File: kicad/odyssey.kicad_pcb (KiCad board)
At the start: 2 copper layers, 33.6 x 18 mm, 7 parts, among them U1 ALS31313KLEATR, U2 MPU-6050, U3 MS560702BA03-50, U4 RP2040, U5 TF-01A

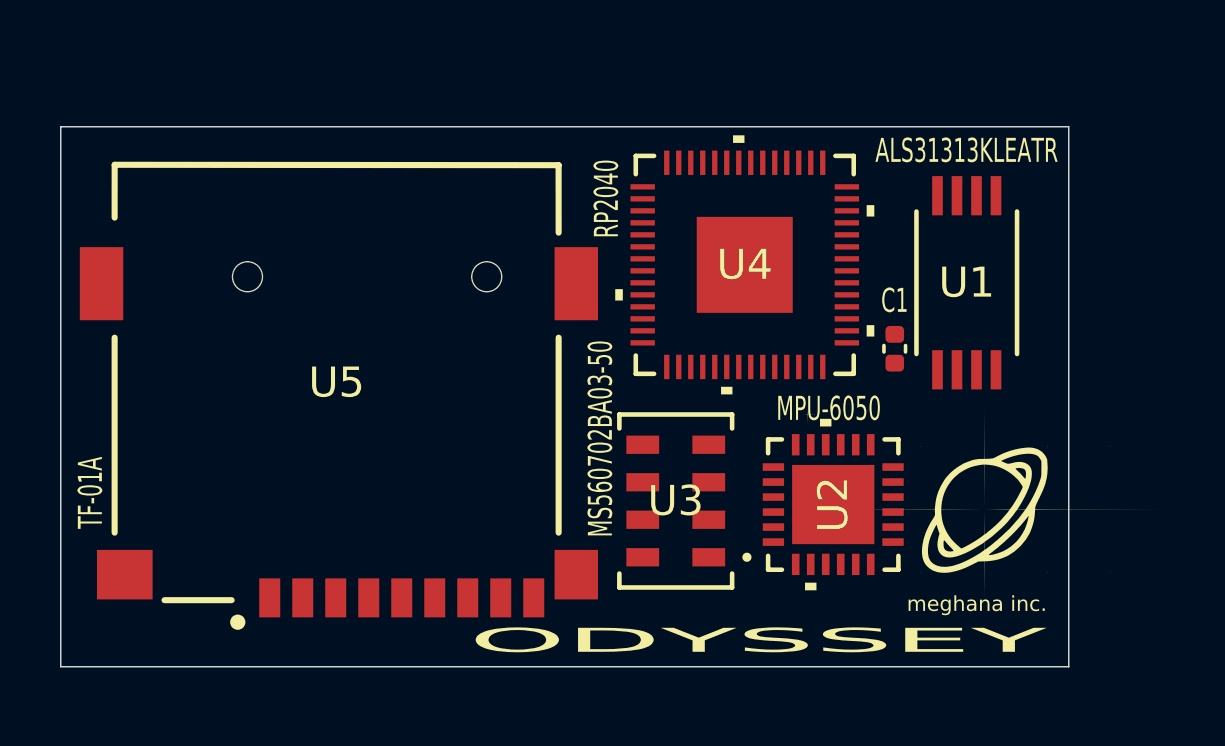
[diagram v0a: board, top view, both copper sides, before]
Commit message: trying firmware stuff
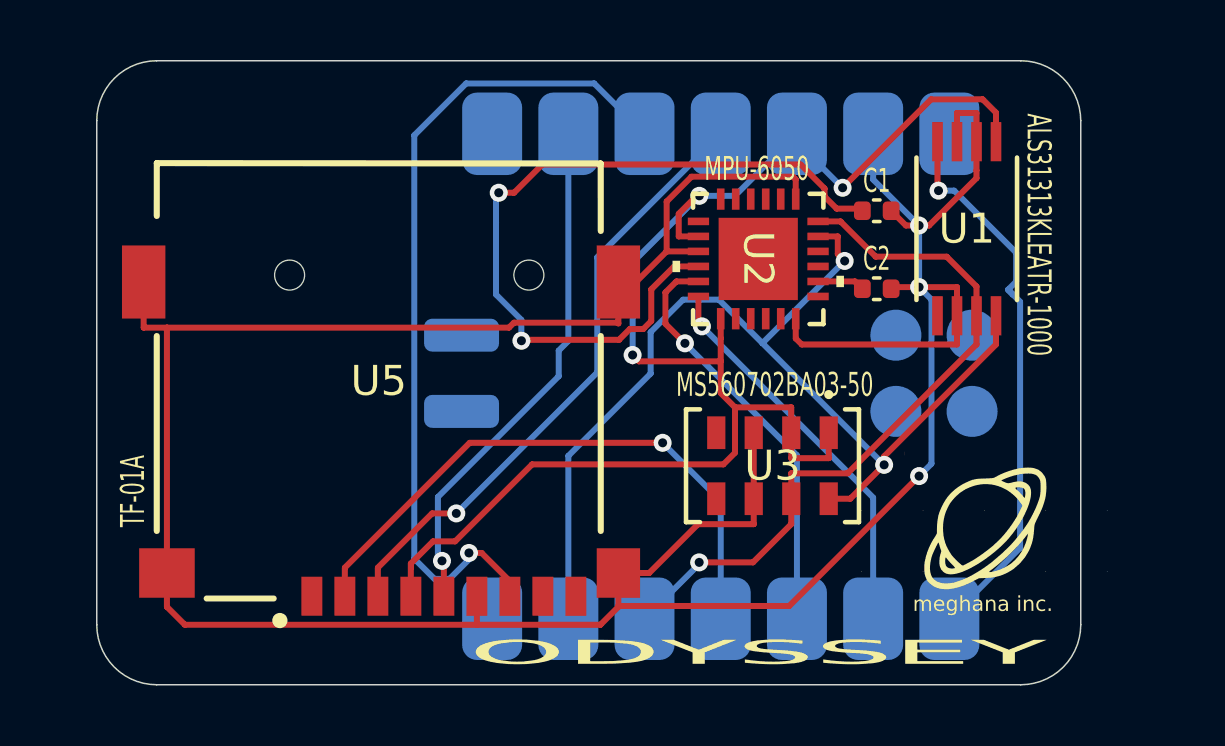
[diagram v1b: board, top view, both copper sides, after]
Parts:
- added C2: C, Capacitor_SMD:C_0402_1005Metric, F.Cu at (163.6, 103.2)
- U1: value ALS31313KLEATR -> ALS31313KLEATR-1000
- U4: value RP2040 -> XIAO-RP2040-SMD; footprint footprints:IC57_RP2040 -> footprints:XIAO-RP2040-SMD; moved to B.Cu
- moved U2 8.56 mm to (159.6, 102.2), turned to -90 degrees
- moved C1 4.64 mm to (163.6, 100.6), turned to 180 degrees
- moved U4 3.88 mm to (158.4, 106.2), turned to 90 degrees
- moved U3 3.43 mm to (160.1, 109.1), turned to -90 degrees
- moved U1 1.80 mm to (166.6, 101.2), turned to -90 degrees
- moved U5 1.40 mm to (147.0, 106.3)
- moved G*** 1.00 mm to (167.8, 111.2)
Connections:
- U1 pad 2: unconnected-(U1-ADR0-Pad2) -> GND
- U1 pad 6: unconnected-(U1-ADR1-Pad6) -> GND
- U2 pad 20: unconnected-(U2-CPOUT-Pad20) -> Net-(U2-CPOUT)
- U2 pad 9: unconnected-(U2-AD0-Pad9) -> GND
- U3 pad 6: unconnected-(U3-SDO-Pad6) -> GND
- U4 pad 1: Net-(U4-IOVDD-Pad1) -> MAGINT
- U4 pad 10: Net-(U4-IOVDD-Pad1) -> MSDMISO
- U4 pad 11: unconnected-(U4-GPIO8-Pad11) -> MSDMOSI
- U4 pad 12: unconnected-(U4-GPIO9-Pad12) -> 3.3V
- U4 pad 13: unconnected-(U4-GPIO10-Pad13) -> GND
- U4 pad 16: MSDCLK -> unconnected-(U4-GND-Pad16)
- U4 pad 17: MSDMISO -> unconnected-(U4-SWDIO-Pad17)
- U4 pad 18: MSDMOSI -> unconnected-(U4-SWDCLK-Pad18)
- U4 pad 2: SDA -> GYROINT
- U4 pad 3: SCL -> GYROFSYNC
- U4 pad 4: MAGINT -> MSDCD
- U4 pad 5: GYROINT -> SDA
- U4 pad 6: GYROFSYNC -> SCL
- U4 pad 7: CD -> unconnected-(U4-GPIO0_D6_TX-Pad7)
- U4 pad 9: unconnected-(U4-GPIO7-Pad9) -> MSDCLK
- U5 pad 2: CD -> MSDCD
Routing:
- net GND: track 0.00 -> 106.5 mm, vias 0 -> 3
- net 3.3V: track 0.00 -> 50.5 mm, vias 0 -> 3
- net SCL: track 0.00 -> 35.5 mm, vias 0 -> 2
- net MSDMISO: track 0.00 -> 28.0 mm, vias 0 -> 1
- net Net-(U2-REGOUT): track 0.00 -> 26.2 mm, vias 0 -> 2
- net SDA: track 0.00 -> 24.0 mm, vias 0 -> 1
- net MSDMOSI: track 0.00 -> 20.6 mm, vias 0 -> 1
- net MSDCD: track 0.00 -> 19.9 mm, vias 0 -> 1
- net MAGINT: track 0.00 -> 18.8 mm, vias 0 -> 1
- net MSDCLK: track 0.00 -> 17.3 mm, vias 0 -> 1
- net GYROFSYNC: track 0.00 -> 14.0 mm, vias 0 -> 1
- net GYROINT: track 0.00 -> 13.2 mm, vias 0 -> 1
- net Net-(U2-CPOUT): track 0.00 -> 1.58 mm
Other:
- board size 33.6 x 18 mm -> 32.8 x 20.8 mm
